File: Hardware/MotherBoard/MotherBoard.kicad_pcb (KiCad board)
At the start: 2 copper layers, 170 x 170 mm, 69 parts, among them J1 USB_OTG, J10 IRQ5, J11 IRQ4, J14 PORT1, J16 PORT2, J17 PORT3, J18 PORT4/ROM, J19 GPIO1, J2 POWER +12V, J20 GPIO2, J21 GPIO1_PWR, J22 GPIO3, J23 GPIO4, J24 GPIO2_PWR, J3 CLOCK_SEL, J4 EXTRN_CLCK, J5 NMI, J6 DMA, J7 IRQ2, J8 IRQ3, J9 IRQ6, SW1 CLOCK_SPD, SW2 OFF_ON, SW3 RESET, U1 74HC590A, U2 AMS1117-5.0, U3 AS6C62256, U4 WD65C02, U5 74HC148, U6 74HC574, U7 ATF22V10B, U8 WD65C22, U9 WD65C22, X1 ACO-16MHz

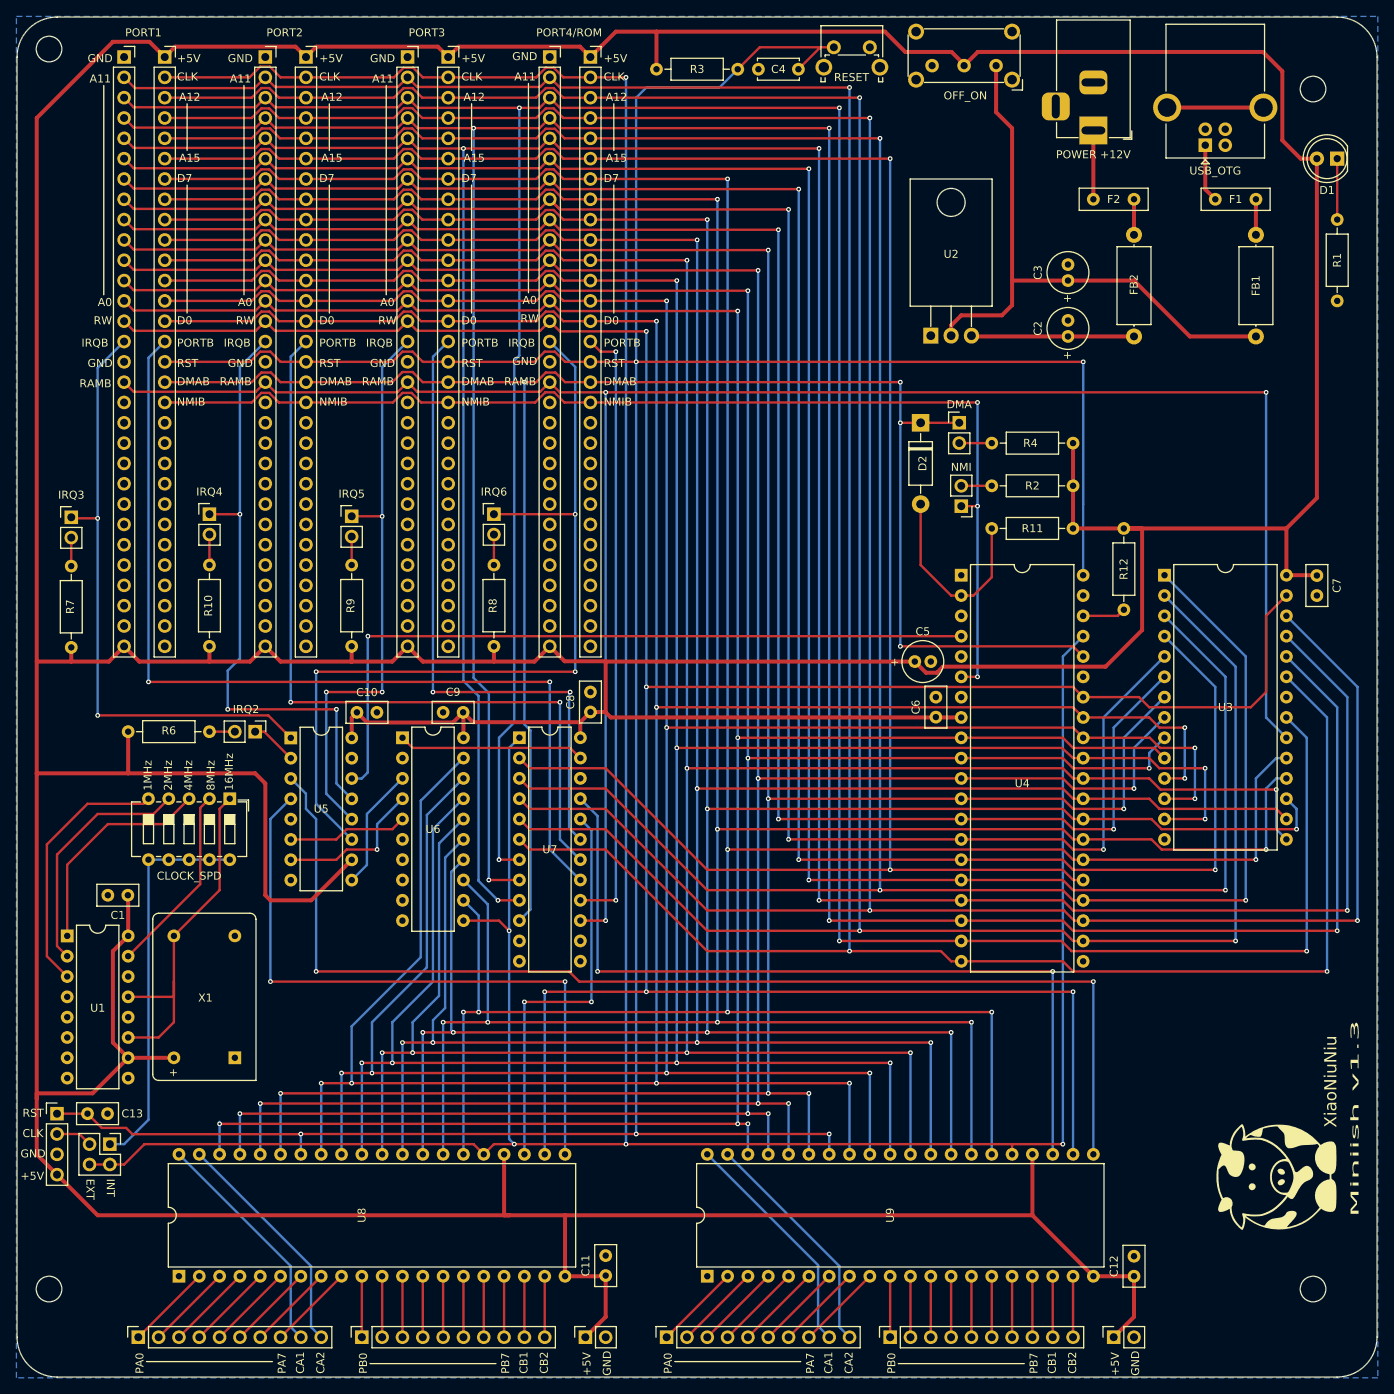
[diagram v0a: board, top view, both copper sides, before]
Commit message: A lot of new hardware
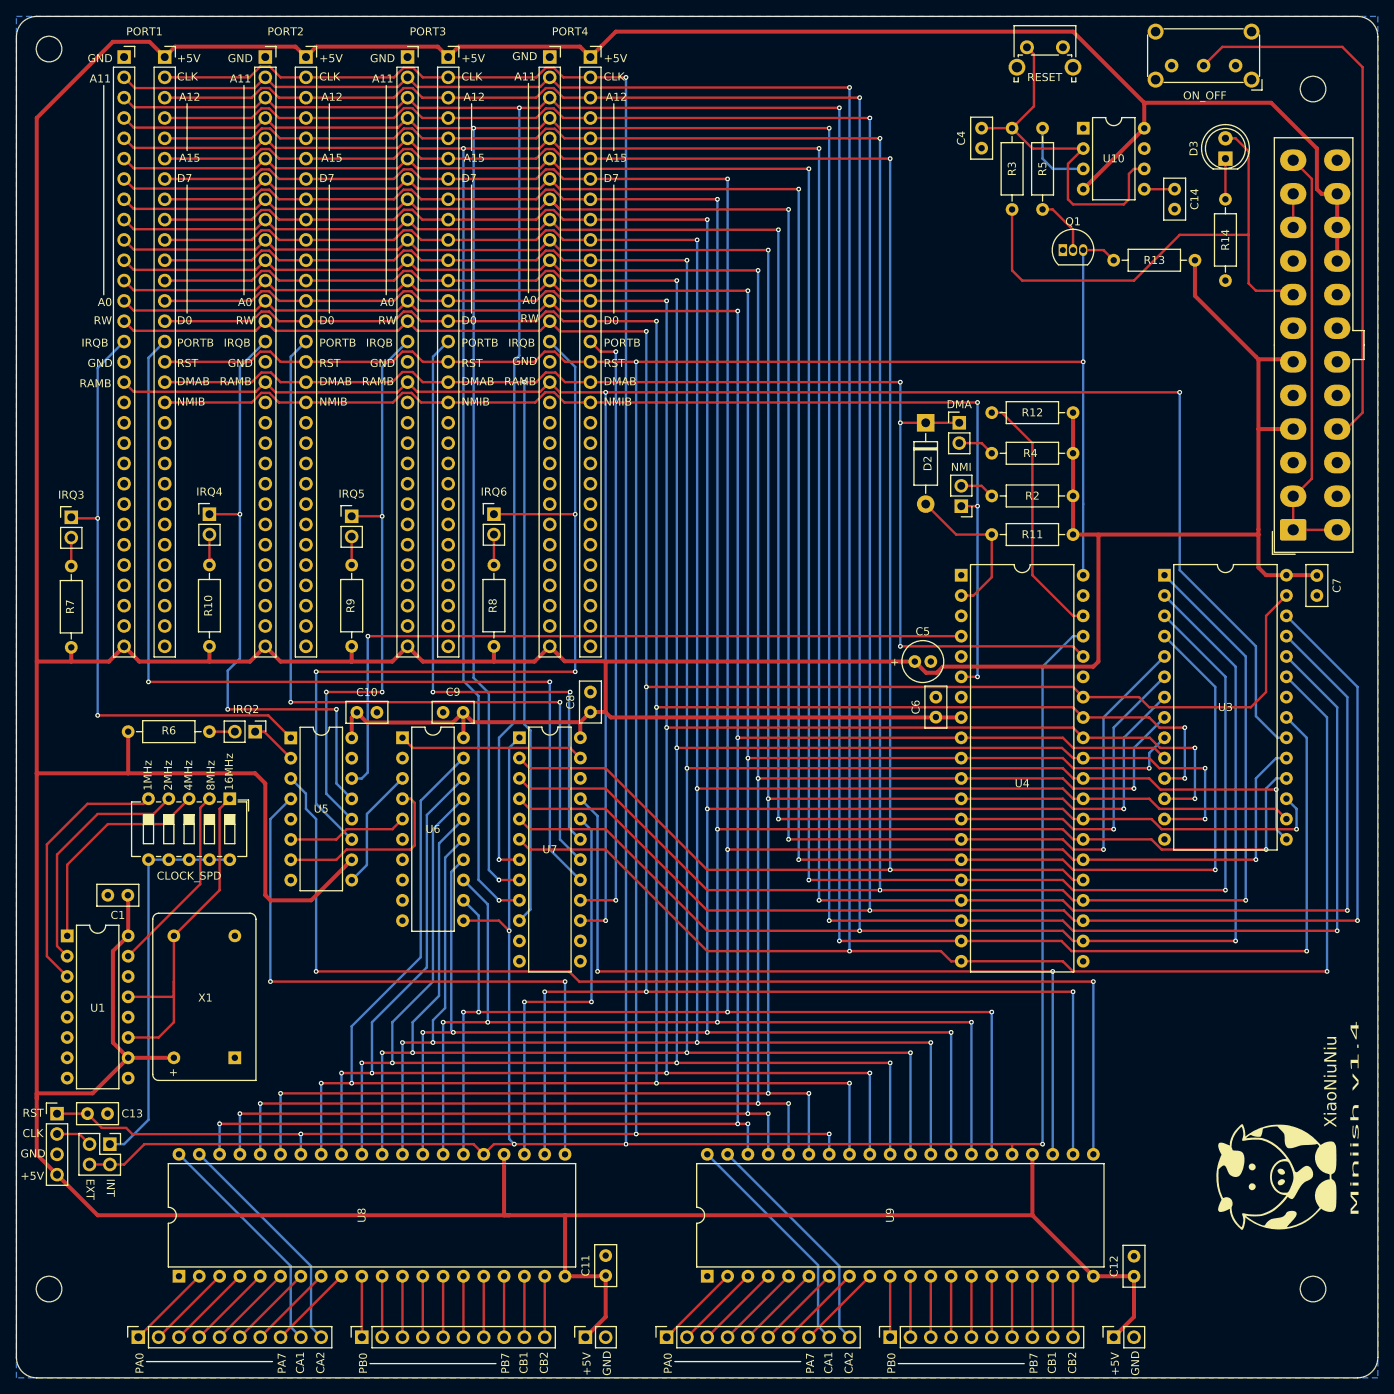
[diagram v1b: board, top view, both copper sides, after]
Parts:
- removed C2: 10uF, Capacitor_THT:C_Radial_D5.0mm_H11.0mm_P2.00mm
- removed C3: 22uF, Capacitor_THT:C_Radial_D5.0mm_H11.0mm_P2.00mm
- removed D1: LED, LED_THT:LED_D5.0mm
- removed F1, F2: 500mA, Resistor_THT:R_Box_L8.4mm_W2.5mm_P5.08mm
- removed FB1, FB2: 100 @ 100MHz, Inductor_THT:L_Axial_L9.5mm_D4.0mm_P12.70mm_Horizontal_Fastron_SMCC
- removed J1: USB_OTG, Connector_USB:USB_B_OST_USB-B1HSxx_Horizontal
- removed J2: POWER +12V, Connector_BarrelJack:BarrelJack_Horizontal
- removed R1: 220, Resistor_THT:R_Axial_DIN0207_L6.3mm_D2.5mm_P10.16mm_Horizontal
- removed U2: AMS1117-5.0, Package_TO_SOT_THT:TO-220-3_Horizontal_TabDown
- added C14: 10nF, Capacitor_THT:C_Disc_D5.0mm_W2.5mm_P2.50mm, F.Cu at (157.8, 36.2)
- added D3: LED, LED_THT:LED_D5.0mm, F.Cu at (164.2, 32.3)
- added J25: ATX-24, Connector_Molex:Molex_Mini-Fit_Jr_5566-24A_2x12_P4.20mm_Vertical, F.Cu at (172.6, 78.7)
- added Q1: 2N3904, Package_TO_SOT_THT:TO-92_Inline, F.Cu at (143.8, 43.8)
- added R13: 10K, Resistor_THT:R_Axial_DIN0207_L6.3mm_D2.5mm_P10.16mm_Horizontal, F.Cu at (150.2, 45.0)
- added R14: 220, Resistor_THT:R_Axial_DIN0207_L6.3mm_D2.5mm_P10.16mm_Horizontal, F.Cu at (164.2, 37.4)
- added R5: 4.7K, Resistor_THT:R_Axial_DIN0207_L6.3mm_D2.5mm_P10.16mm_Horizontal, F.Cu at (141.3, 28.5)
- added U10: NE555P, Package_DIP:DIP-8_W7.62mm, F.Cu at (146.4, 28.5)
- C4: value 470nF -> 100nF; footprint Capacitor_THT:C_Disc_D5.0mm_W2.5mm_P5.00mm -> Capacitor_THT:C_Disc_D5.0mm_W2.5mm_P2.50mm
- J14, J16, J17, J18: footprint NESConnector:NES_Cartdrige -> Connector_NES:NES_Cartdrige
- R3: value 10K -> 1M
- SW2: value OFF_ON -> ON_OFF
- moved R3 47.8 mm to (137.5, 38.7), turned to 90 degrees
- moved SW2 29.9 mm to (165.4, 20.7)
- moved R12 29.7 mm to (134.9, 64.1), turned to 0 degrees
- moved SW3 24.1 mm to (139.3, 18.4)
- moved C4 24.1 mm to (133.7, 28.5), turned to -90 degrees
- moved R4 1.27 mm to (134.9, 69.2)
- moved R2 1.27 mm to (134.9, 74.5)
- moved R11 0.76 mm to (134.9, 79.3)
- moved D2 0.63 mm to (126.7, 65.4)
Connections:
- C4 pad 1: RESET -> Net-(U10-THR)
- R3 pad 1: +5V -> PWR_OK
- R3 pad 2: RESET -> Net-(U10-THR)
- SW2 pad 1: Net-(SW2-A) -> GND
- SW2 pad 2: +5V -> Net-(J25-PS_ON#)
- SW3 pad 1: RESET -> Net-(U10-THR)
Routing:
- net Net-(SW2-A): track 73.8 -> 0.00 mm
- net Net-(J25-PS_ON#): track 0.00 -> 68.0 mm
- net PWR_OK: track 0.00 -> 65.6 mm
- net unconnected-(J25-+3.3V-Pad1): track 0.00 -> 53.6 mm
- net Net-(U10-THR): track 0.00 -> 46.0 mm
- net RESET: track 408.1 -> 362.1 mm
- net /North Bridge/SOB: track 5.40 -> 31.6 mm
- net Net-(U2-VI): track 19.6 -> 0.00 mm
- net +5V: track 966.3 -> 980.5 mm
- net unconnected-(J1-Shield-Pad5): track 12.0 -> 0.00 mm
- net Net-(U10-Q): track 0.00 -> 9.43 mm
- net Net-(F2-Pad1): track 8.61 -> 0.00 mm
- net Net-(D1-K): track 7.62 -> 0.00 mm
- net Net-(Q1-B): track 0.00 -> 7.40 mm
- net Net-(J1-VBUS): track 7.28 -> 0.00 mm
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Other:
- board size 170 x 170 mm -> 170.2 x 170.2 mm
- board text added: "Miniish v1.4"
- board text removed: "Miniish v1.3"
